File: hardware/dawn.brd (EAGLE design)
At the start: 68.2 x 68.6 mm, 31 parts, among them IC1 ATMEGA328-20P, IC3 DS1307, Q2 16Mhz, Q3 32.768kHz, Q4 BUZ11BV, T3 BC547B, X1 MKDSN1,5/2-5,08, X2 MKDSN1,5/2-5,08

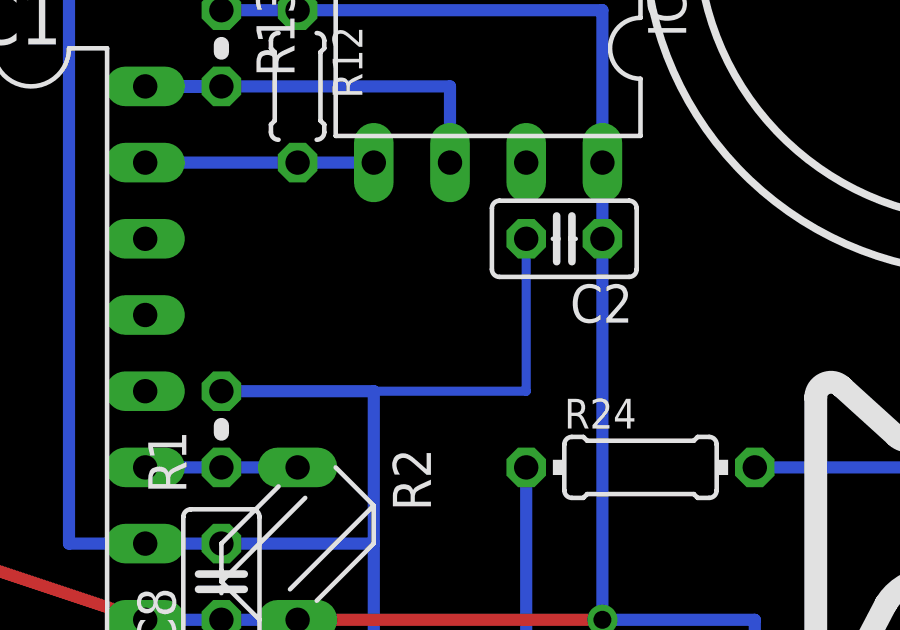
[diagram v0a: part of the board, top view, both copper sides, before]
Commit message: Cleanup.
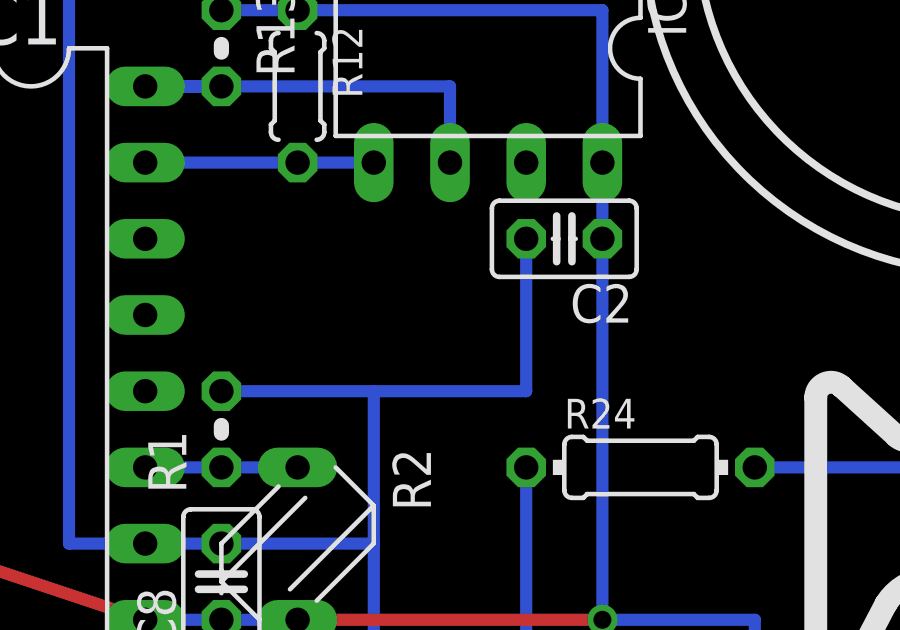
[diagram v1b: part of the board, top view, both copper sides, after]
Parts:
- R1: value 470 -> 100
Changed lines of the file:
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@@
 <element name="JP1" library="pinhead" package="1X05" value="GPIO" x="40.64" y="31.75" rot="R90"/>
 <element name="KK1" library="heatsink" package="PF752" value="PF750" x="86.36" y="52.07"/>
-<element name="R1" library="rcl" package="0204V" value="470" x="55.88" y="50.8" rot="R90"/>
+<element name="R1" library="rcl" package="0204V" value="100" x="55.88" y="50.8" rot="R90"/>
 <element name="R2" library="ptc-ntc" package="B57164" value="1k" x="58.42" y="46.99" rot="R270">
 <attribute name="OC_NEWARK" value="29M3118" x="58.42" y="46.99" size="1.778" layer="27" rot="R270" display="off"/>
@@
 <wire x1="60.96" y1="52.07" x2="60.96" y2="46.99" width="0.4064" layer="16"/>
 <contactref element="C2" pad="2"/>
-<wire x1="66.04" y1="57.15" x2="66.04" y2="52.07" width="0.3048" layer="16"/>
-<wire x1="66.04" y1="52.07" x2="60.96" y2="52.07" width="0.3048" layer="16"/>
+<wire x1="66.04" y1="57.15" x2="66.04" y2="52.07" width="0.4064" layer="16"/>
+<wire x1="66.04" y1="52.07" x2="60.96" y2="52.07" width="0.4064" layer="16"/>
 </signal>
 <signal name="N$13">
